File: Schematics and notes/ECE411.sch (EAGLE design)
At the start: 24 parts, among them J1 POWER_JACK, J2 AVR_SPI_PROG_3X2NS, J3 6_PIN_SERIAL_CABLEPTH, U1 328P, U2 LM358

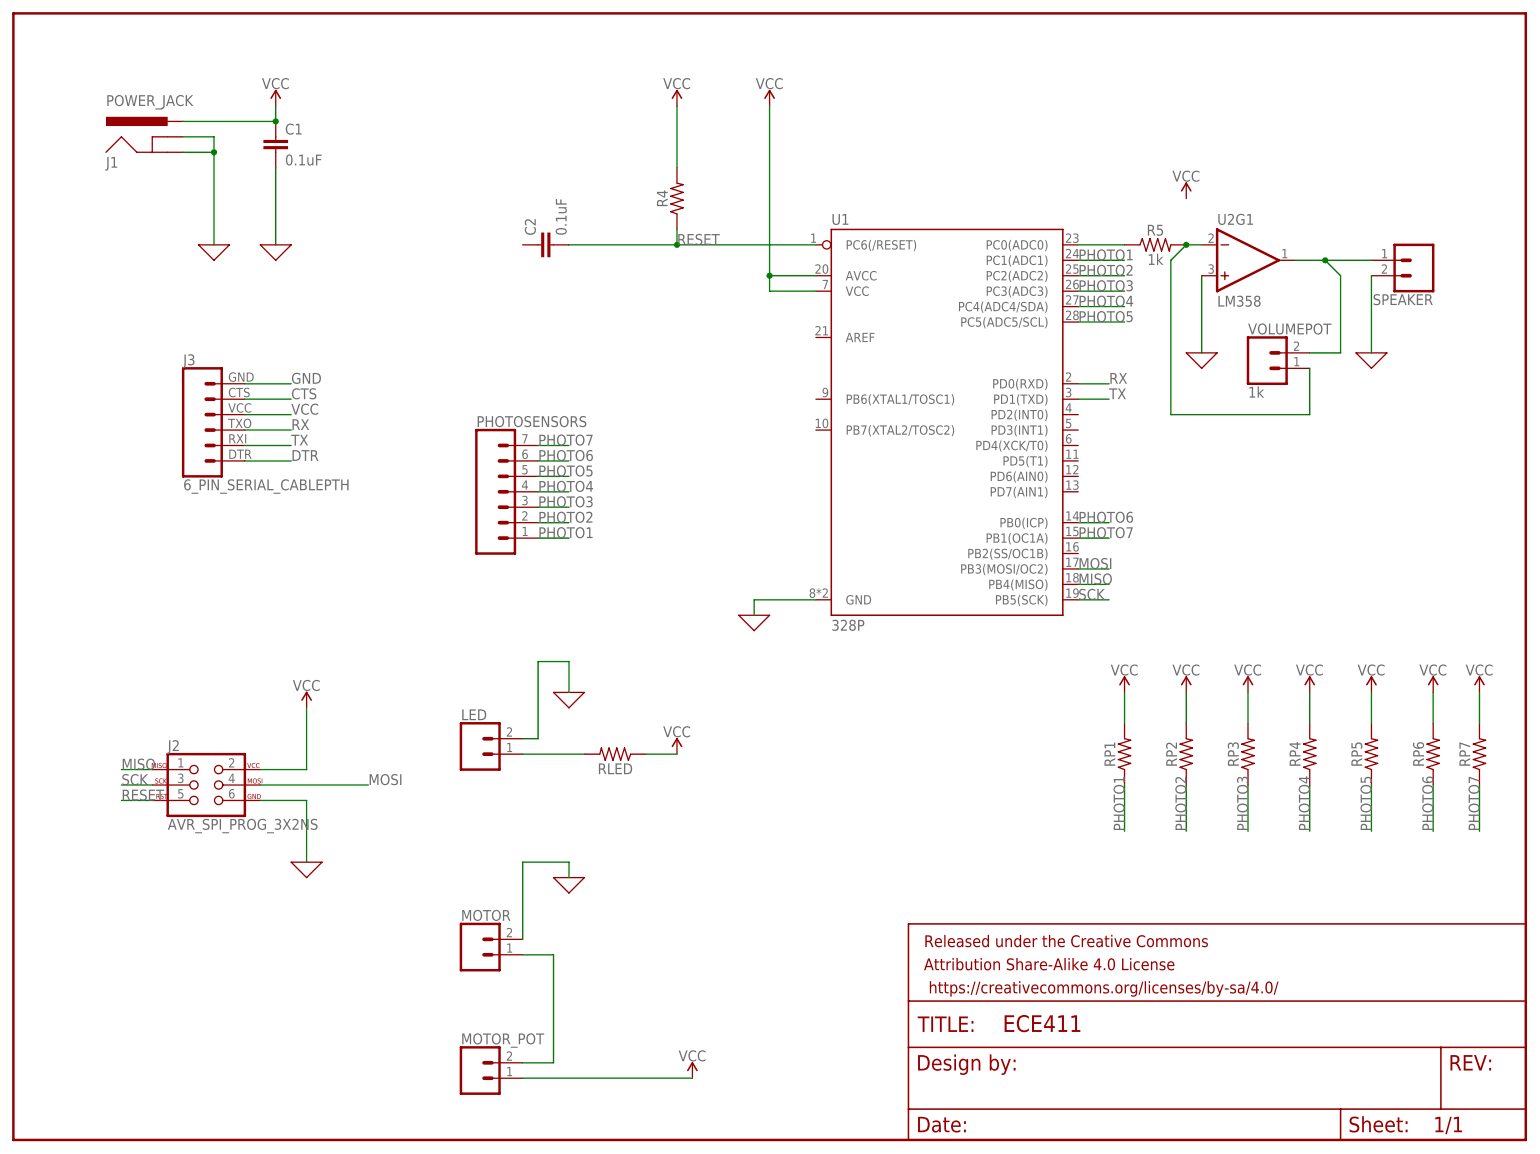
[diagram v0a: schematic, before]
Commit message: Add files via upload
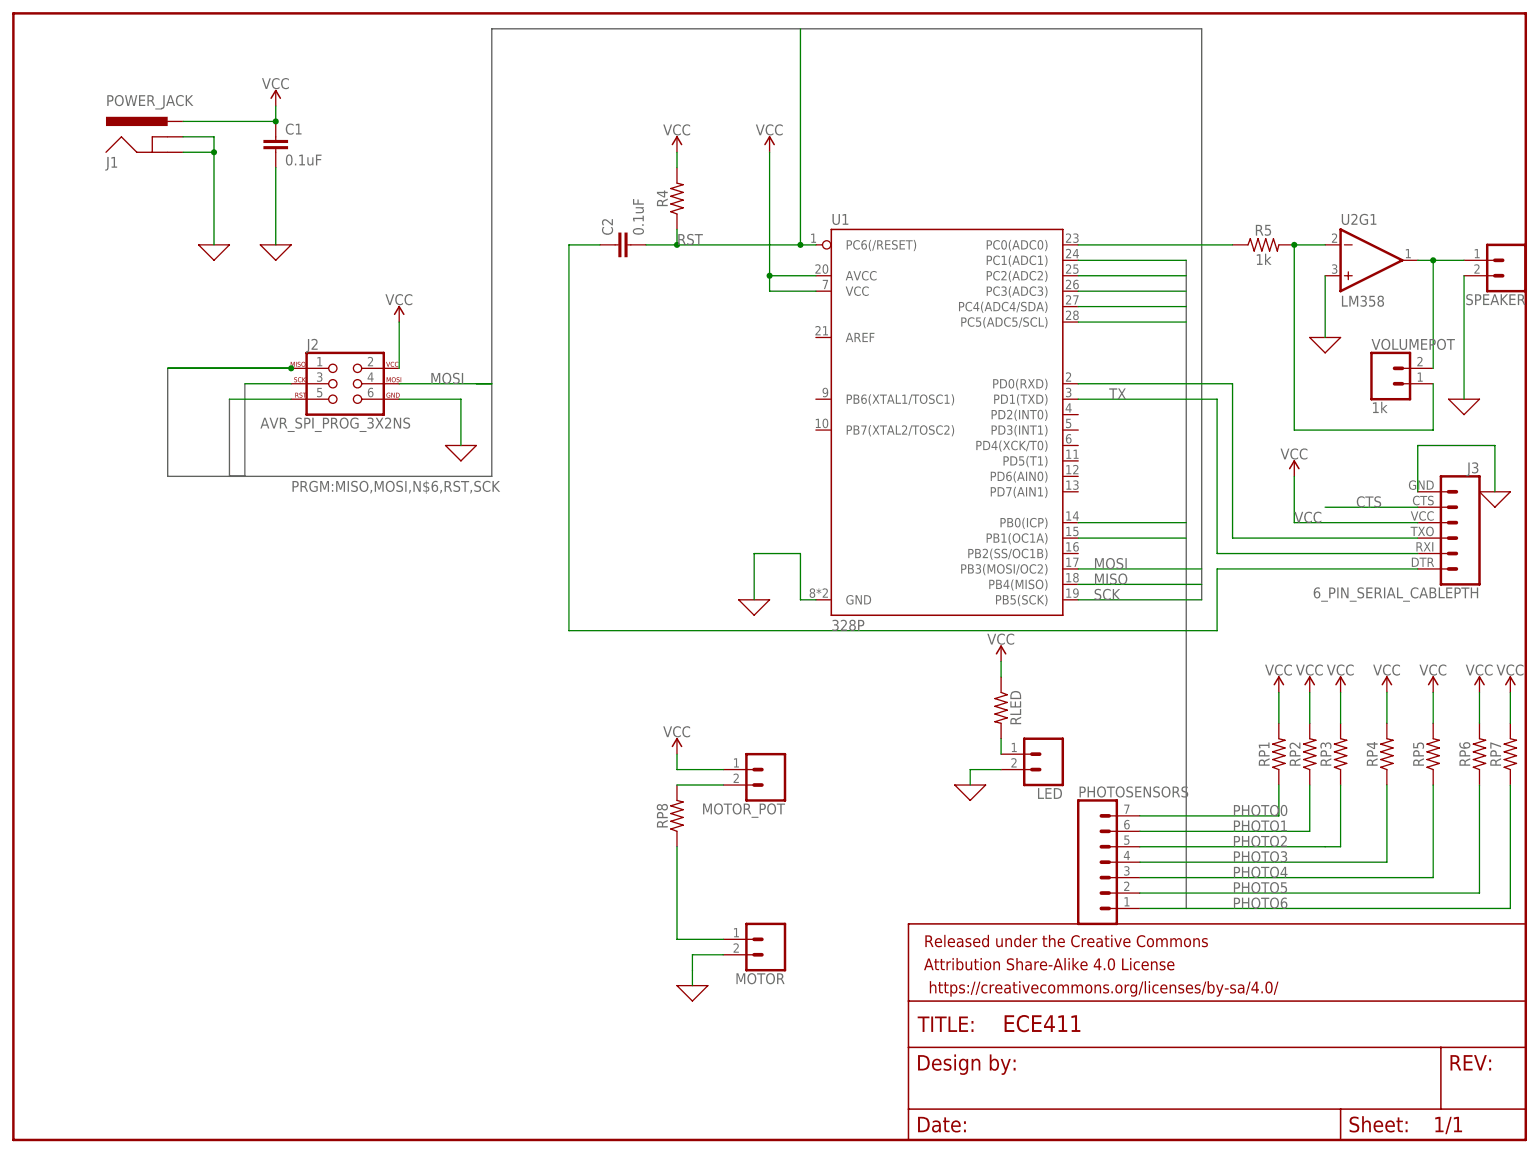
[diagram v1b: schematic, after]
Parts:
- added RP8: (no value), SparkFun-Resistors:RESISTOR0603
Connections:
- net RESET renamed RST
- net RX renamed N$4
- removed net DTR: J3.1
- removed net GND: J3.6
- removed net PHOTO7: PHOTOSENSORS.7, RP7.1, U1.PB1(OC1A)
- new net N$5: C2.1, J3.1
- new net N$7: MOTOR.1, RP8.1
- new net PHOTO0: PHOTOSENSORS.7, RP1.1, U1.PC1(ADC1)
- net 0: now also J3.6
- net N$2: now also RP8.2; no longer MOTOR.1
- net PHOTO1: now also PHOTOSENSORS.6, RP2.1, U1.PC2(ADC2); no longer PHOTOSENSORS.1, RP1.1, U1.PC1(ADC1)
- net PHOTO2: now also PHOTOSENSORS.5, RP3.1, U1.PC3(ADC3); no longer PHOTOSENSORS.2, RP2.1, U1.PC2(ADC2)
- net PHOTO3: now also PHOTOSENSORS.4, RP4.1, U1.PC4(ADC4/SDA); no longer PHOTOSENSORS.3, RP3.1, U1.PC3(ADC3)
- net PHOTO4: now also PHOTOSENSORS.3, RP5.1, U1.PC5(ADC5/SCL); no longer PHOTOSENSORS.4, RP4.1, U1.PC4(ADC4/SDA)
- net PHOTO5: now also PHOTOSENSORS.2, RP6.1, U1.PB0(ICP); no longer PHOTOSENSORS.5, RP5.1, U1.PC5(ADC5/SCL)
- net PHOTO6: now also PHOTOSENSORS.1, RP7.1, U1.PB1(OC1A); no longer PHOTOSENSORS.6, RP6.1, U1.PB0(ICP)
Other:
- moved on the sheet: C2, J2, J3, LED, MOTOR, MOTOR_POT, PHOTOSENSORS, R5, RLED, RP1, RP2, RP3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
